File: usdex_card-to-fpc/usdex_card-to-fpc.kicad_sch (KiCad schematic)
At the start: 2 parts, among them J1 Micro_SDex_PCB, J2 Conn_01x16_Socket

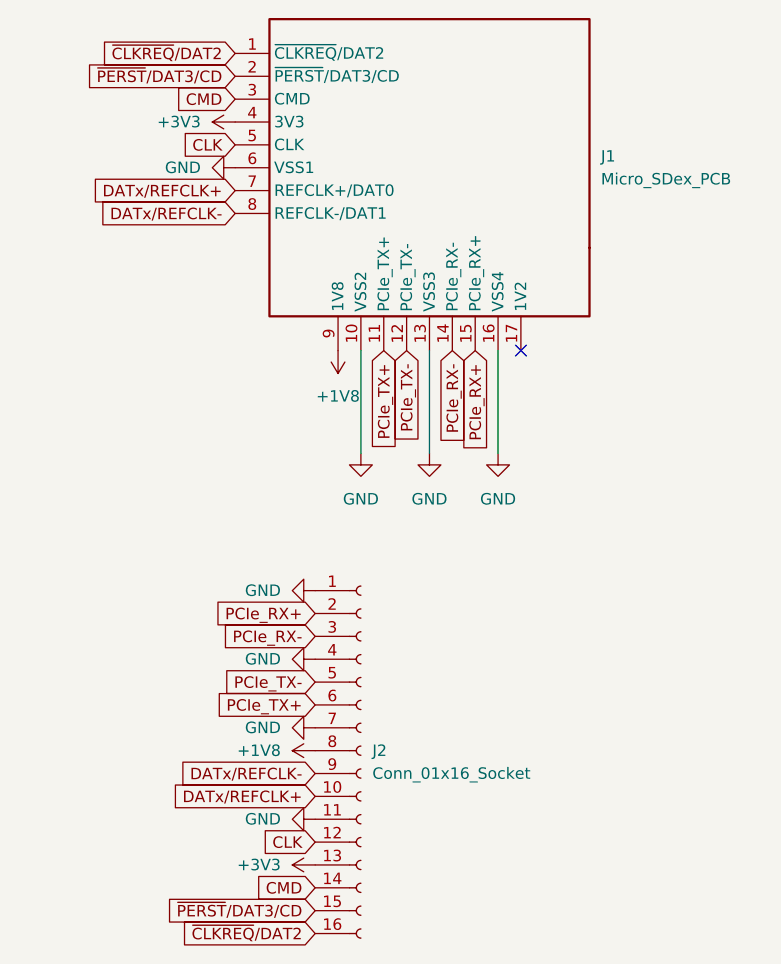
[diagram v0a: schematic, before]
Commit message: finish usdex card
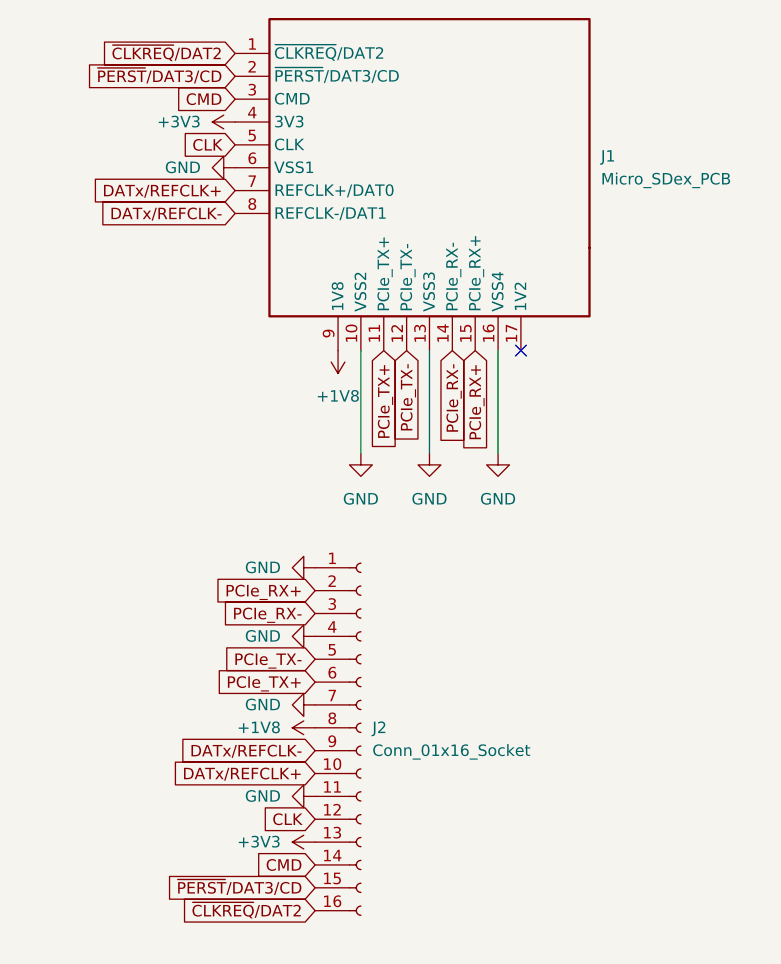
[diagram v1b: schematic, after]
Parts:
- J2: footprint m1cha:usdex-fpc-1x16-0.64mm -> m1cha:usdex-fpc-1x18-0.55mm
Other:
- moved on the sheet: J2
